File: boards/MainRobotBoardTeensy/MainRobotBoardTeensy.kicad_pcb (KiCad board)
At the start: 2 copper layers, 174 x 121.1 mm, 162 parts, among them J1 Screw_Terminal_01x02, J10 B4B-XH-A, J11 IDC, J2 B3B-XH-A, J3 B3B-XH-A, J5 B3B-XH-A, J6 B3B-XH-A, J7 B3B-XH-A, J8 B3B-XH-A, J9 B3B-XH-A, Q1 AO3400A, Q10 AO3400A, Q11 AO3400A, Q12 AO3400A, Q13 AO3400A, Q14 AO3400A, Q15 AO3400A, Q16 AO3400A, Q17 AO3400A, Q18 AO3400A, Q19 AO3400A, Q2 AO3400A, Q20 AO3400A, Q3 AO3400A, Q4 AO3400A, Q5 AO3400A, Q6 AO3400A, Q9 AO3400A, U1 Teensy4.1, U10 KWL-R1025BB, U11 SSD1306, U2 TLC555CDR, U3 SN74HC08DR, U4 SN74HC08DR, U5 74HCT125D, U6 SN74HC08DR, U7 ACS37220, U8 SSD1306, U9 74HCT125D

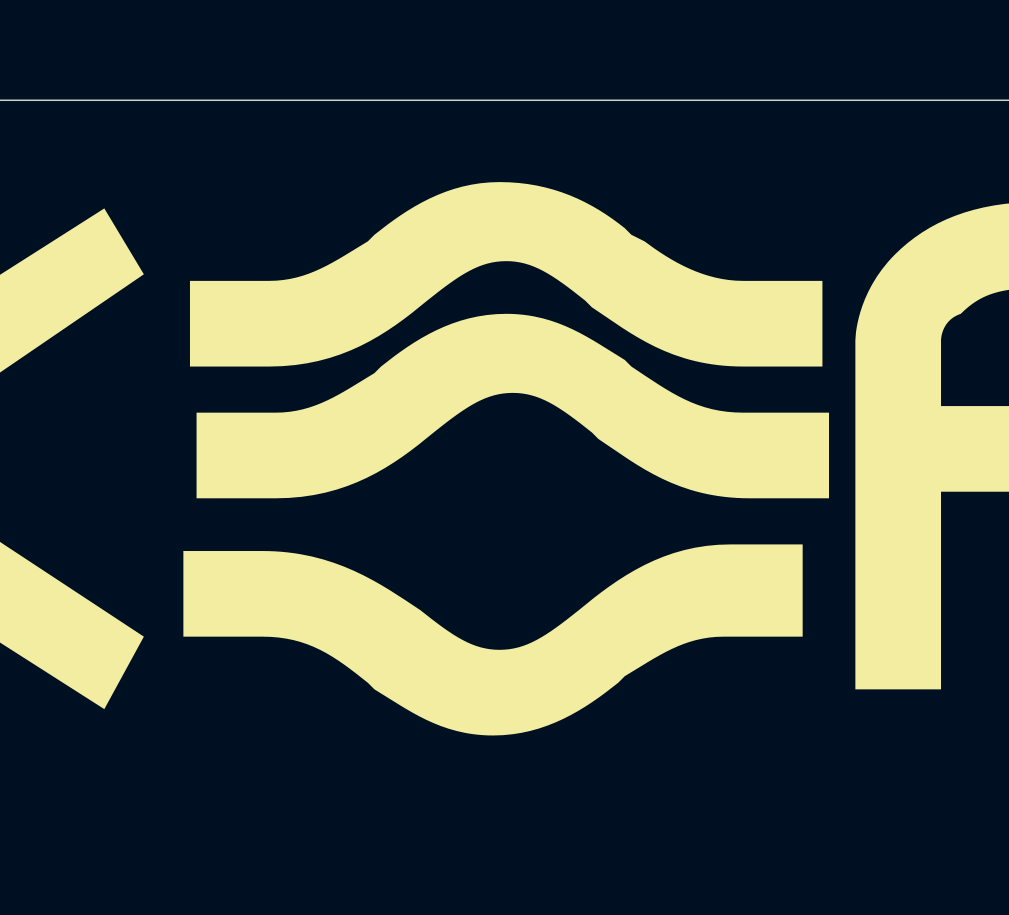
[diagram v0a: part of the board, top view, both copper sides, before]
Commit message: Re-finalize audio board and cleanup
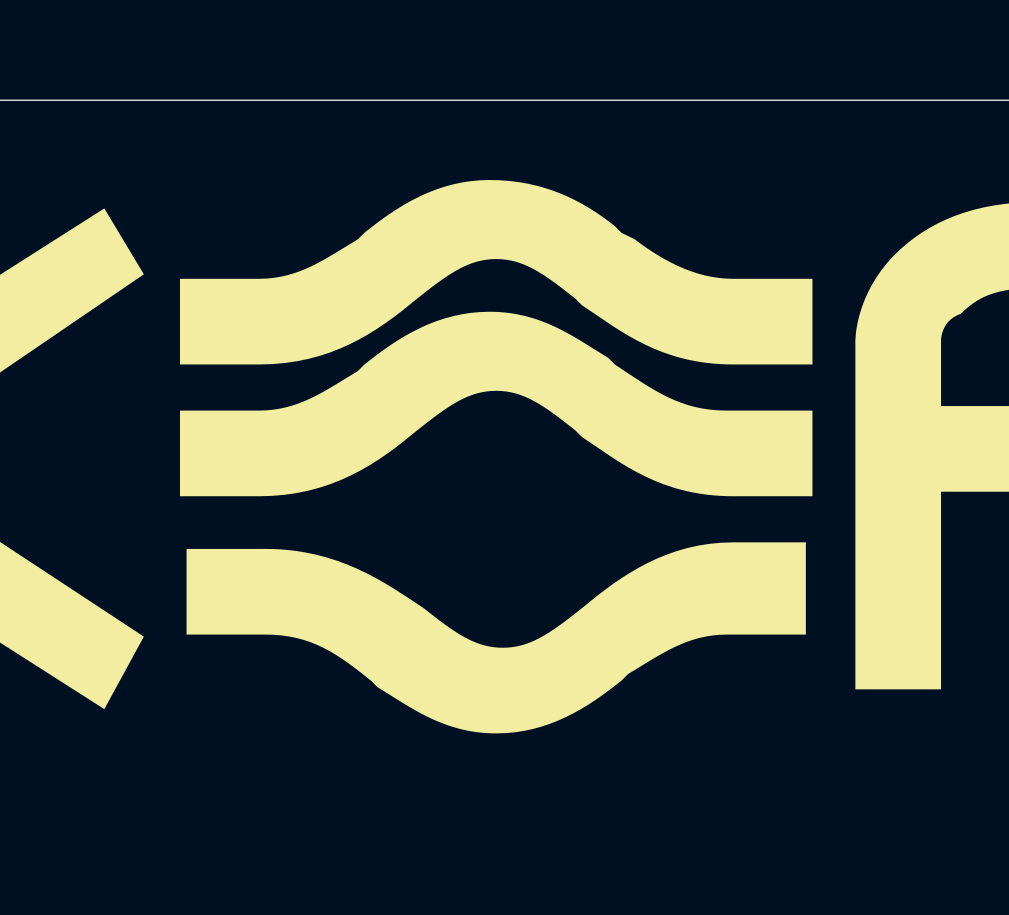
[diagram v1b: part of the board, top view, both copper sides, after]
